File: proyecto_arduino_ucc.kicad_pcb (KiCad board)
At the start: 2 copper layers, 14 parts, among them J1 USB_A, J2 Header, U1 ATtiny85-20S

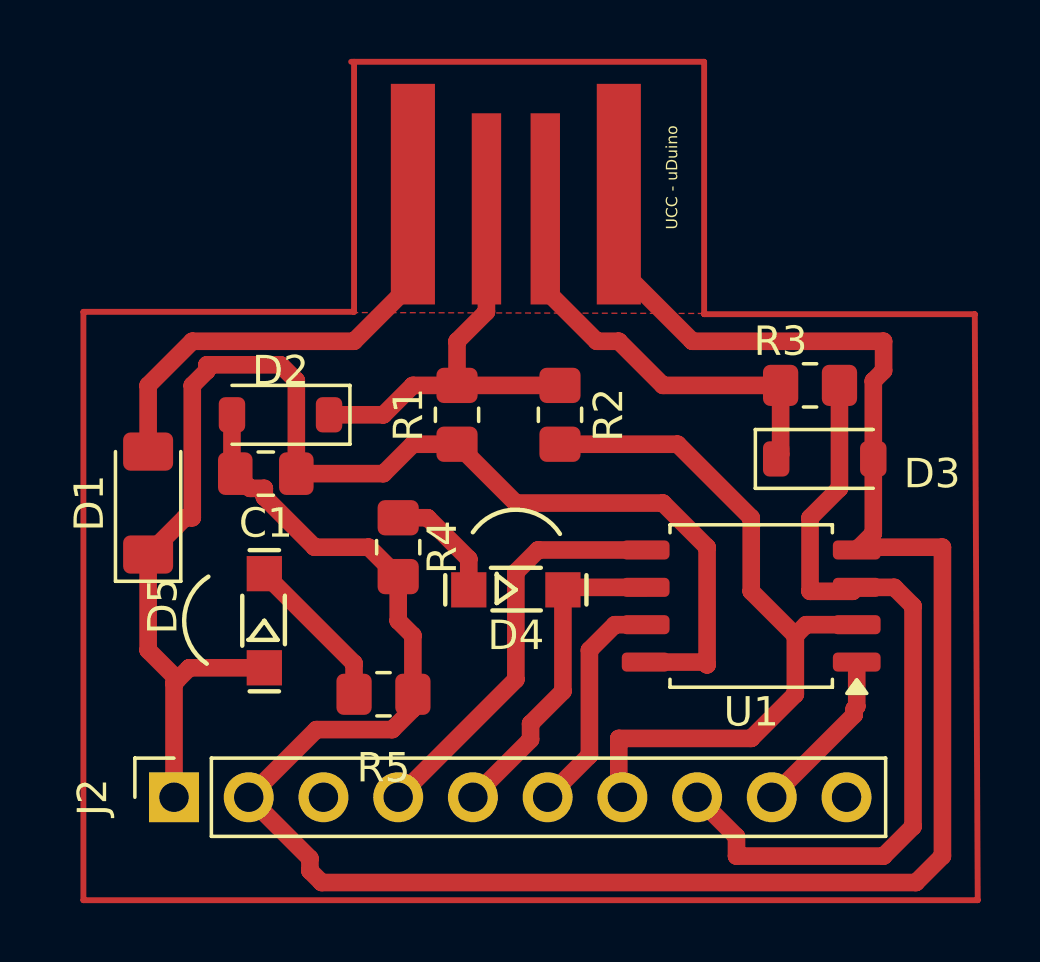
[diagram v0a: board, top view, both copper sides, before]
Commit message: Add files via upload
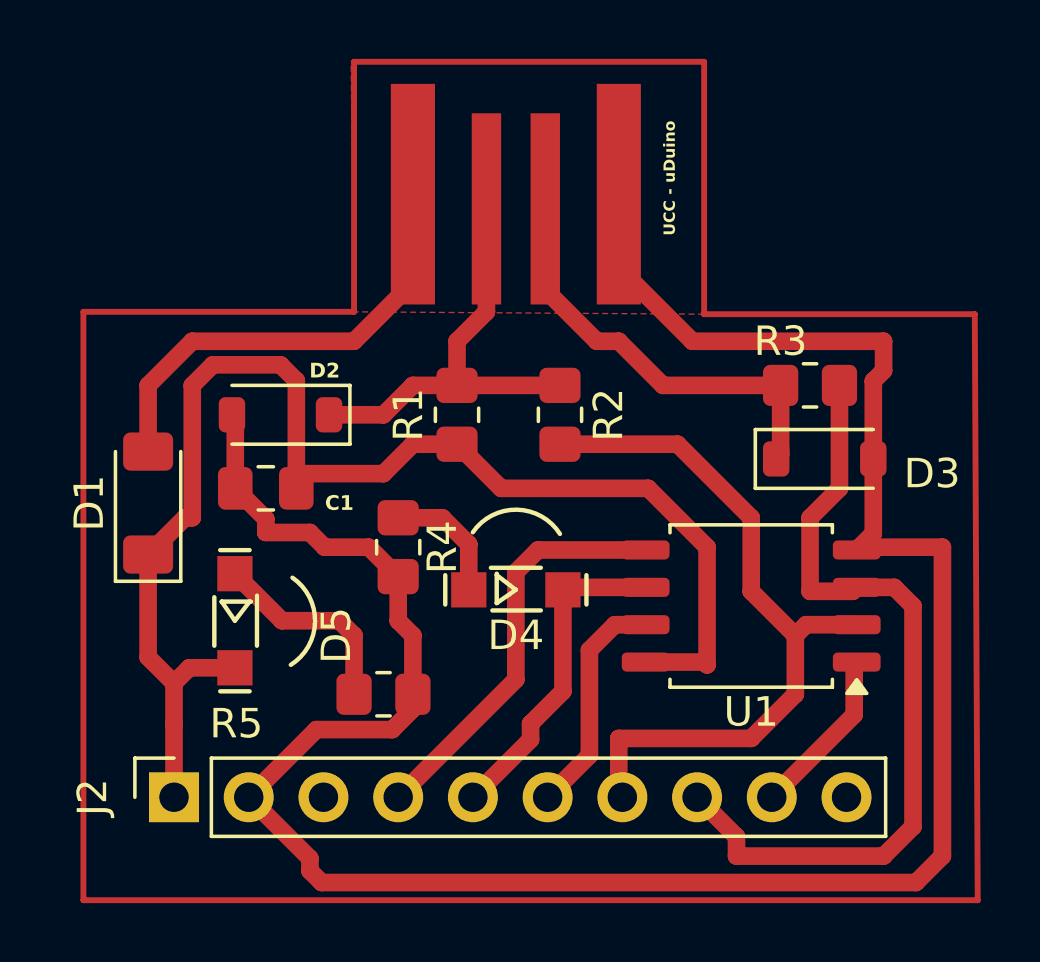
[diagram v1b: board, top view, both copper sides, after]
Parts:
- moved D5 1.00 mm to (136.4, 107.0), turned to -90 degrees
- moved C1 0.50 mm to (137.0, 102.0)
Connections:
- D5 pad 1: +1V5 -> Net-(D5-A)
- D5 pad 2: Net-(D5-A) -> +1V5
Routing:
- net Net-(D5-A): track 5.36 -> 6.92 mm
- net +1V5: track 47.9 -> 46.9 mm

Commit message: Add files via upload
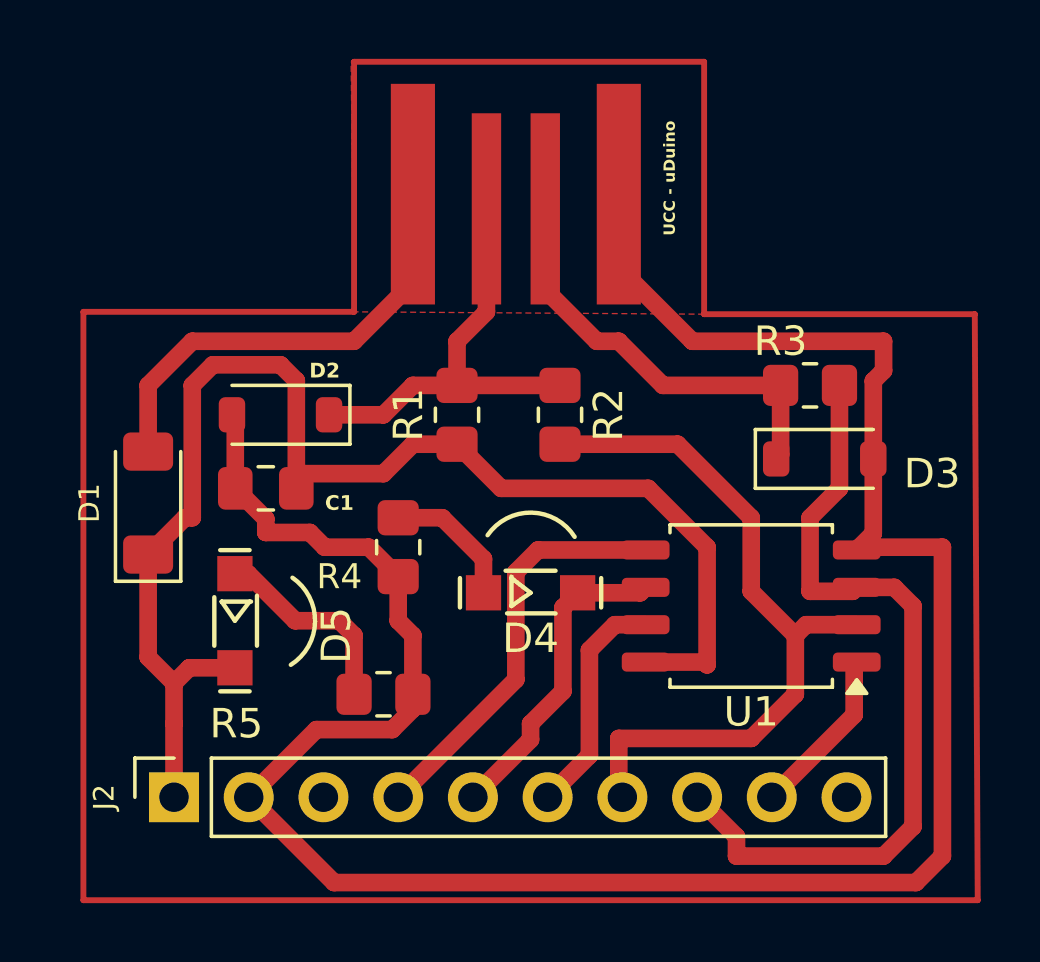
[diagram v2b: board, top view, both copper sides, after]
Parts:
- moved D4 0.51 mm to (146.5, 105.1)
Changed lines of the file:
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@@
 	(footprint "Huellas-UCC:LED.R"
 		(layer "F.Cu")
-		(at 146 105)
+		(at 146.5 105.1)
 		(property "Reference" "D4"
 			(at -0.5 2 0)
@@
 		(tags "Through hole socket strip THT 1x10 2.54mm single row")
 		(property "Reference" "J2"
-			(at 0 -2.77 90)
+			(at 0 -2.38 90)
 			(layer "F.SilkS")
 			(effects
 				(font
-					(size 1 1)
-					(thickness 0.15)
+					(size 0.7 0.7)
+					(thickness 0.1)
 				)
 			)
@@
 			(net 11 "unconnected-(J2-Pin_3-Pad3)")
 			(pinfunction "Pin_3")
-			(pintype "passive")
+			(pintype "passive+no_connect")
 		)
 		(pad "4" thru_hole circle
@@
 			(net 10 "unconnected-(J2-Pin_10-Pad10)")
 			(pinfunction "Pin_10")
-			(pintype "passive")
+			(pintype "passive+no_connect")
 		)
 		(embedded_fonts no)
@@
 		(tags "resistor handsolder")
 		(property "Reference" "R4"
-			(at 0 -1.5 90)
+			(at 1 2 180)
 			(layer "F.SilkS")
 			(effects
 				(font
-					(size 1 1)
+					(size 0.85 0.85)
 					(thickness 0.15)
 				)
@@
 			(effects
 				(font
-					(size 1 1)
-					(thickness 0.15)
+					(size 0.7 0.7)
+					(thickness 0.1)
 				)
 			)
@@
 	)
 	(segment
-		(start 143.5 100.5)
-		(end 145 102)
+		(start 133 107.74)
+		(end 133 104.25)
 		(width 0.6)
 		(layer "F.Cu")
@@
 	)
 	(segment
-		(start 133.88 108.62)
-		(end 134.4 108.1)
+		(start 143.5 100.5)
+		(end 145 102)
 		(width 0.6)
 		(layer "F.Cu")
@@
 	)
 	(segment
-		(start 135.95 108.1)
+		(start 133.88 108.62)
 		(end 134.4 108.1)
 		(width 0.6)
@@
 	)
 	(segment
-		(start 151.905 107.905)
-		(end 149.9125 107.905)
+		(start 134.4 108.1)
+		(end 135.95 108.1)
 		(width 0.6)
 		(layer "F.Cu")
@@
 	)
 	(segment
-		(start 133 107.74)
-		(end 133 104.25)
+		(start 151.905 107.905)
+		(end 149.9125 107.905)
 		(width 0.6)
 		(layer "F.Cu")
@@
 	)
 	(segment
-		(start 157.1825 104)
-		(end 160 104)
+		(start 142 109)
+		(end 142 107)
 		(width 0.6)
 		(layer "F.Cu")
@@
 	)
 	(segment
-		(start 142 109)
-		(end 142 107)
+		(start 160 114.5)
+		(end 160 104)
 		(width 0.6)
 		(layer "F.Cu")
@@
 	)
 	(segment
+		(start 159.1 115.4)
+		(end 160 114.5)
+		(width 0.6)
+		(layer "F.Cu")
+		(net 3)
+	)
+	(segment
 		(start 136.42 112.5)
 		(end 138.719 110.201)
@@
 	)
 	(segment
+		(start 160 104)
+		(end 157.1825 104)
+		(width 0.6)
+		(layer "F.Cu")
+		(net 3)
+	)
+	(segment
 		(start 137 103.5)
 		(end 137 103.0375)
@@
 	)
 	(segment
-		(start 160 114.5)
-		(end 159.101 115.399)
-		(width 0.6)
-		(layer "F.Cu")
-		(net 3)
-	)
-	(segment
 		(start 138.719 110.201)
 		(end 141.299 110.201)
@@
 	)
 	(segment
-		(start 160 104)
-		(end 160 114.5)
-		(width 0.6)
-		(layer "F.Cu")
-		(net 3)
-	)
-	(segment
 		(start 157.65 98.35)
 		(end 157.65 101)
@@
 	)
 	(segment
-		(start 138.5 114.58)
-		(end 136.42 112.5)
-		(width 0.6)
-		(layer "F.Cu")
-		(net 3)
-	)
-	(segment
 		(start 135.9625 102)
 		(end 135.9625 99.6125)
@@
 	)
 	(segment
-		(start 158 97)
-		(end 158 98)
+		(start 139.32 115.4)
+		(end 159.1 115.4)
 		(width 0.6)
 		(layer "F.Cu")
@@
 	)
 	(segment
-		(start 140.5 104)
-		(end 139 104)
+		(start 158 97)
+		(end 158 98)
 		(width 0.6)
 		(layer "F.Cu")
@@
 	)
 	(segment
-		(start 159.101 115.399)
-		(end 138.899 115.399)
+		(start 140.5 104)
+		(end 139 104)
 		(width 0.6)
 		(layer "F.Cu")
@@
 	)
 	(segment
-		(start 157.0875 104.095)
-		(end 157.1825 104)
-		(width 0.6)
-		(layer "F.Cu")
-		(net 3)
-	)
-	(segment
 		(start 141.5 106.5)
 		(end 141.5 105)
@@
 	)
 	(segment
-		(start 139 104)
-		(end 138.5 103.5)
+		(start 136.42 112.5)
+		(end 139.32 115.4)
 		(width 0.6)
 		(layer "F.Cu")
@@
 	)
 	(segment
-		(start 138.899 115.399)
-		(end 138.5 115)
+		(start 139 104)
+		(end 138.5 103.5)
 		(width 0.6)
 		(layer "F.Cu")
@@
 	)
 	(segment
-		(start 138.5 115)
-		(end 138.5 114.58)
+		(start 157.1825 104)
+		(end 157.0875 104.095)
 		(width 0.6)
 		(layer "F.Cu")
@@
 	)
 	(segment
-		(start 147.1 105.45)
-		(end 147.1 108.9)
+		(start 147.1 108.9)
+		(end 147.1 106.05)
 		(width 0.6)
 		(layer "F.Cu")
@@
 	)
 	(segment
-		(start 149.9125 105.365)
-		(end 147.185 105.365)
+		(start 146 110.54)
+		(end 144.04 112.5)
 		(width 0.6)
 		(layer "F.Cu")
@@
 	)
 	(segment
-		(start 146 110.54)
-		(end 144.04 112.5)
+		(start 146 110)
+		(end 146 110.54)
 		(width 0.6)
 		(layer "F.Cu")
@@
 	)
 	(segment
-		(start 146 110)
-		(end 146 110.54)
+		(start 149.7275 105.55)
+		(end 149.9125 105.365)
 		(width 0.6)
 		(layer "F.Cu")
@@
 	)
 	(segment
-		(start 147.185 105.365)
-		(end 147.1 105.45)
+		(start 147.1 106.05)
+		(end 147.6 105.55)
 		(width 0.6)
 		(layer "F.Cu")
@@
 	)
 	(segment
-		(start 143.9 105.45)
-		(end 143.9 103.9)
+		(start 147.6 105.55)
+		(end 149.7275 105.55)
+		(width 0.6)
+		(layer "F.Cu")
+		(net 12)
+	)
+	(segment
+		(start 144.4 104.4)
+		(end 144.4 105.55)
 		(width 0.6)
 		(layer "F.Cu")
@@
 	(segment
 		(start 143 103)
-		(end 141.5 103)
+		(end 144.4 104.4)
 		(width 0.6)
 		(layer "F.Cu")
@@
 	)
 	(segment
-		(start 143.9 103.9)
+		(start 141.5 103)
 		(end 143 103)
 		(width 0.6)
@@
 	)
 	(segment
-		(start 139.5 106.5)
-		(end 137.55 106.5)
+		(start 140 109)
+		(end 140 107)
 		(width 0.6)
 		(layer "F.Cu")
@@
 	)
 	(segment
-		(start 140 109)
-		(end 140 107)
+		(start 140 107)
+		(end 139.5 106.5)
 		(width 0.6)
 		(layer "F.Cu")
@@
 	)
 	(segment
-		(start 140 107)
+		(start 138 106.5)
 		(end 139.5 106.5)
 		(width 0.6)
@@
 	)
 	(segment
-		(start 137.55 106.5)
-		(end 135.95 104.9)
+		(start 135.95 104.9)
+		(end 136.4 104.9)
+		(width 0.6)
+		(layer "F.Cu")
+		(net 14)
+	)
+	(segment
+		(start 136.4 104.9)
+		(end 138 106.5)
 		(width 0.6)
 		(layer "F.Cu")
@@
 			)
 		)
+	)
+	(zone
+		(net 0)
+		(net_name "")
+		(layer "Edge.Cuts")
+		(hatch edge 0.5)
+		(connect_pads
+			(clearance 0.5)
+		)
+		(min_thickness 0.25)
+		(filled_areas_thickness no)
+		(fill
+			(thermal_gap 0.5)
+			(thermal_bridge_width 0.5)
+		)
+		(polygon
+			(pts
+				(xy 131 96) (xy 161 96) (xy 161 116) (xy 131 116)
+			)
+		)
